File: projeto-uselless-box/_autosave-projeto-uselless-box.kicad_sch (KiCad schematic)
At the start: 13 parts, among them J2 Conn_Para_Fita, M1 Motor_Servo, M2 Motor_Servo, M3 Motor_Servo, Q1 TIP41, SW1 SW_DPST_x2, U3 L7812

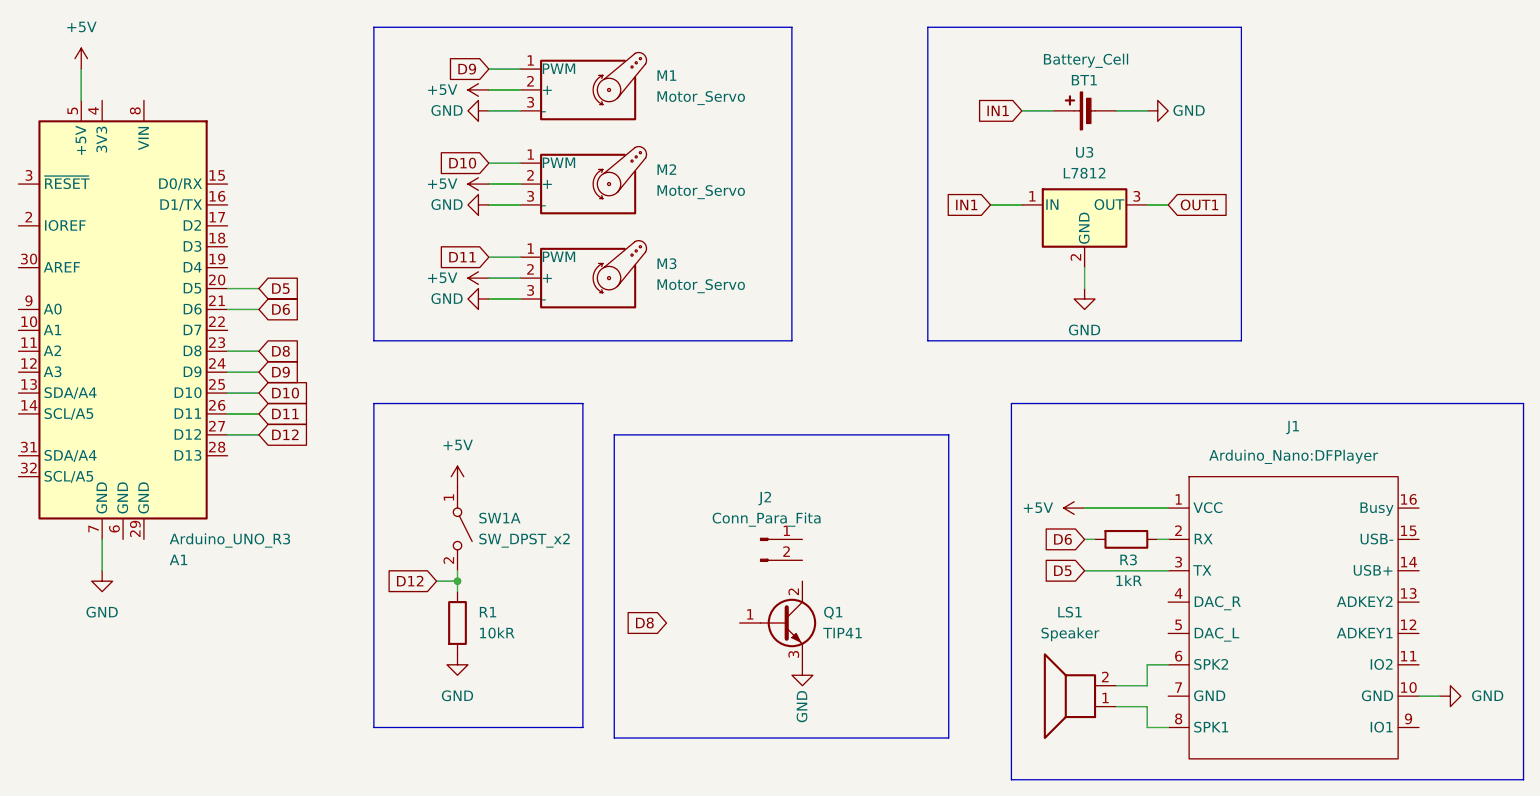
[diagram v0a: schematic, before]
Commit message: Finished the first prototype of PCB
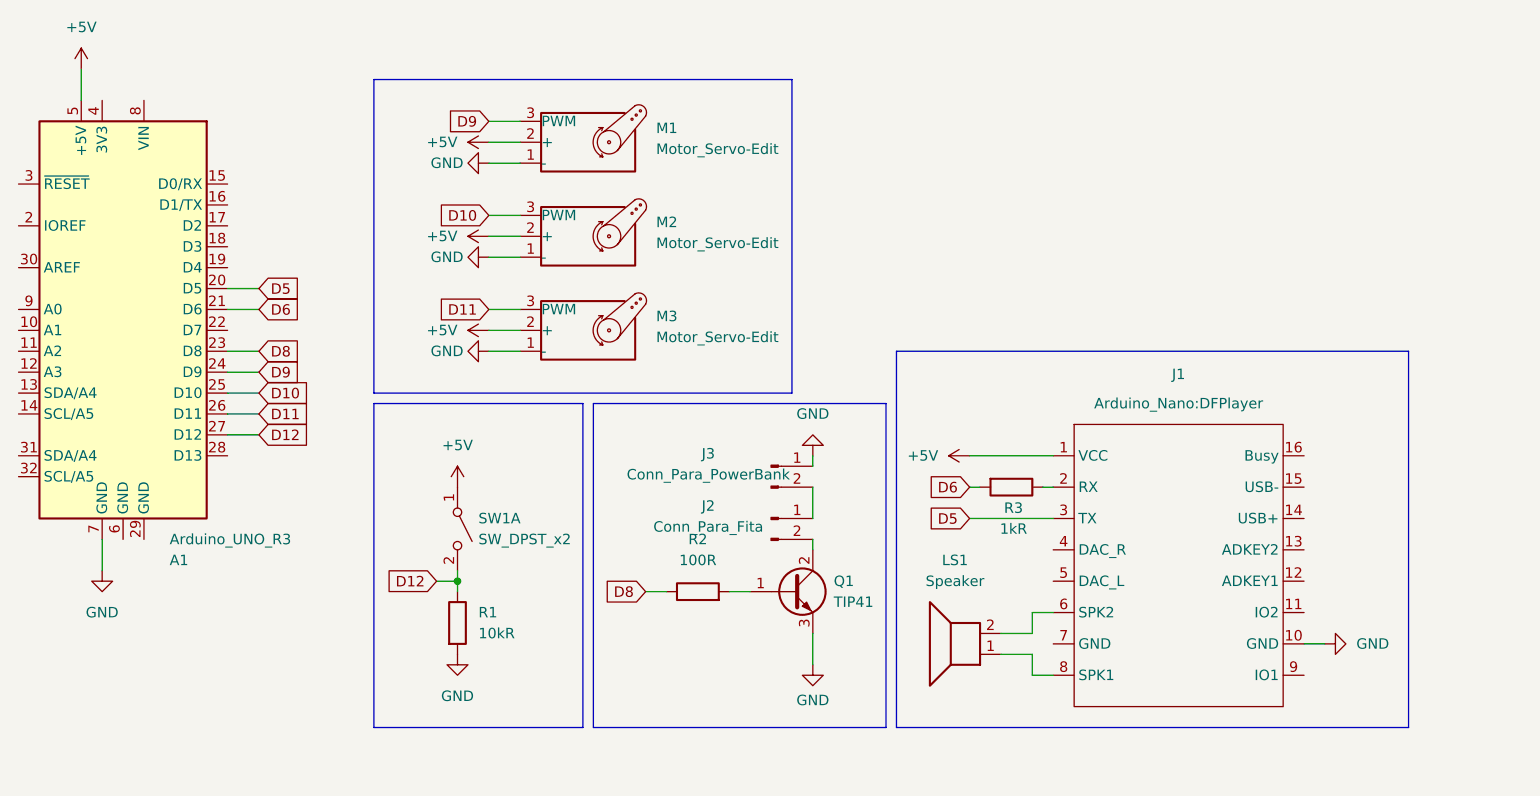
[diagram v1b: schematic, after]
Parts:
- removed BT1: Battery_Cell, symbol Device:Battery_Cell
- removed M1, M2, M3: Motor_Servo, Connector_PinSocket_2.54mm:PinSocket_1x03_P2.54mm_Vertical, symbol Motor:Motor_Servo
- removed U3: L7812, symbol Regulator_Linear:L7812
- added J3: Conn_Para_PowerBank, TerminalBlock_Phoenix:TerminalBlock_Phoenix_MKDS-1,5-2-5.08_1x02_P5.08mm_Horizontal, symbol Connector:Conn_01x02_Pin
- added M1, M2, M3: Motor_Servo-Edit, Connector_PinSocket_2.54mm:PinSocket_1x02_P2.54mm_Vertical, symbol New_Library:Motor_Servo-Edit
- added R2: 100R, Resistor_THT:R_Axial_DIN0207_L6.3mm_D2.5mm_P10.16mm_Horizontal, symbol Device:R
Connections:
- net +5V: now also M1.2 (+), M2.2 (+), M3.2 (+)
- net D10: now also M2.3 (PWM)
- net D11: now also M3.3 (PWM)
- net D8: now also R2.1
- net D9: now also M1.3 (PWM)
- net GND: now also J3.1 (Pin_1), M1.1 (-), M2.1 (-), M3.1 (-)
- net at Q1.1 (B): now also R2.2
- net at Q1.2 (C): now also J2.2 (Pin_2)
- net at J2.1 (Pin_1): now also J3.2 (Pin_2)
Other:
- moved on the sheet: J1, J2, LS1, Q1, R3
